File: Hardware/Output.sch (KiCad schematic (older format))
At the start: 15 parts

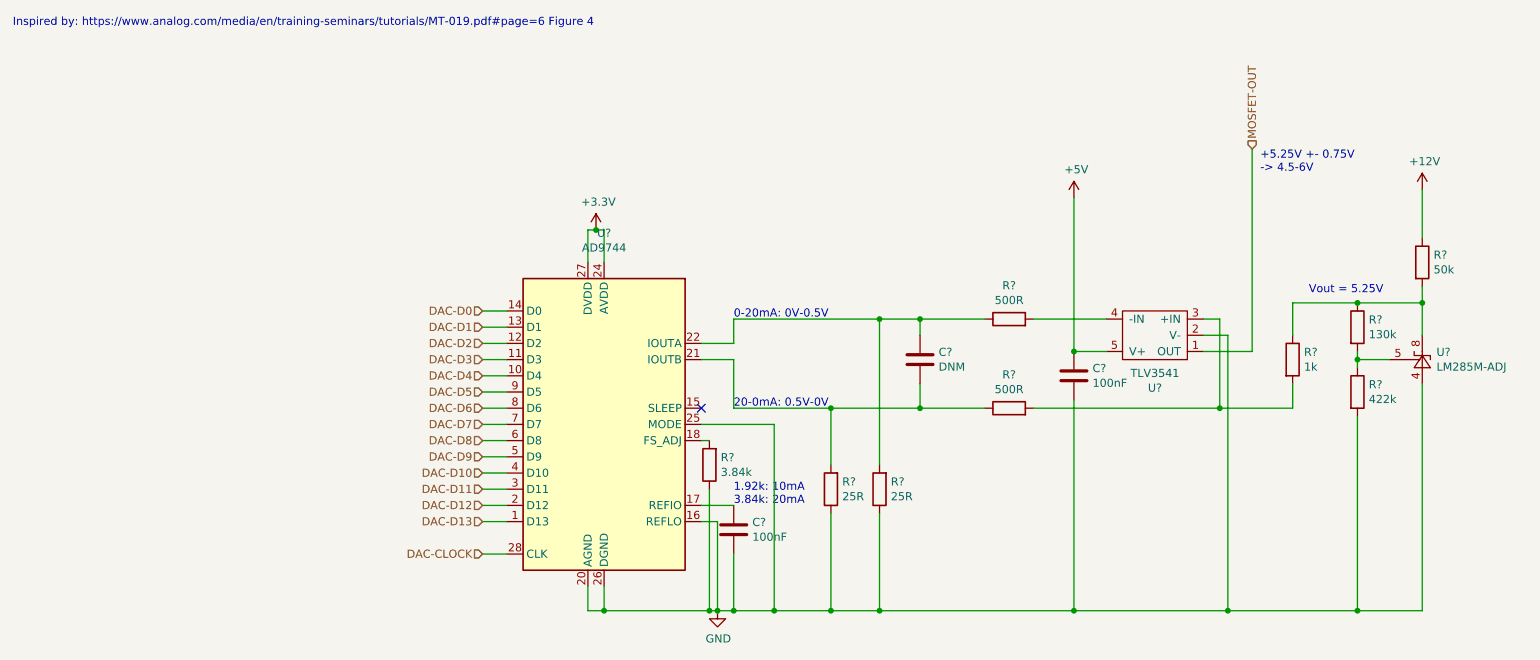
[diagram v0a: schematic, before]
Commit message: output amplifier stage finished+THS3091 added to library
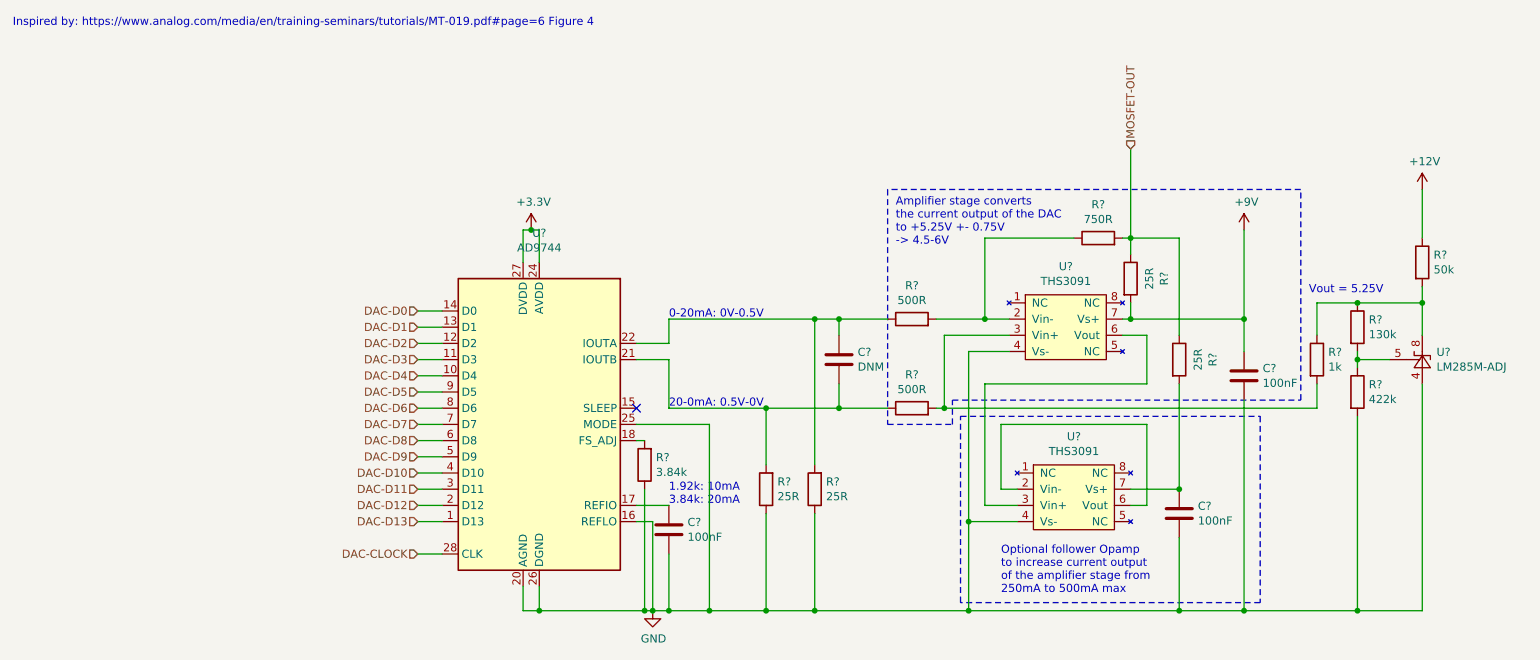
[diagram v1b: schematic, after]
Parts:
- removed U?: TLV3541, symbol OS-LD:TVL3541
- added C?: 100nF, symbol Device:C
- added R?: 750R, symbol Device:R
- added R? (x2): 25R, symbol Device:R
- added U? (x2): THS3091, symbol OS-LD:THS3091
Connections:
- net GND: now also C?.1, U?.4 (Vs-), U?.4 (Vs-)
- net MOSFET-OUT: now also R?.1, R?.1, R?.2
- net at R?.2, R?.2: now also U?.3 (Vin+)
- net at R?.2: now also R?.1, U?.2 (Vin-)
- net +5V renamed +9V
- net +9V: now also R?.2, U?.7 (Vs+)
- new net: U?.3 (Vin+), U?.6 (Vout)
- new net: U?.2 (Vin-), U?.6 (Vout)
- new net: C?.2, R?.2, U?.7 (Vs+)
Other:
- note added: "Amplifier stage converts \nthe current output of the DAC \nto +5.25V +- 0.75V\n-> 4.5-6V"
- note added: "Optional follower Opamp\nto increase current output \nof the amplifier stage from \n250mA to 500mA max"
- note removed: "+5.25V +- 0.75V\n-> 4.5-6V"
- moved on the sheet: C?, R?, U?
